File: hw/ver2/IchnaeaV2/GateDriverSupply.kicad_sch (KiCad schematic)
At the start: 0 parts

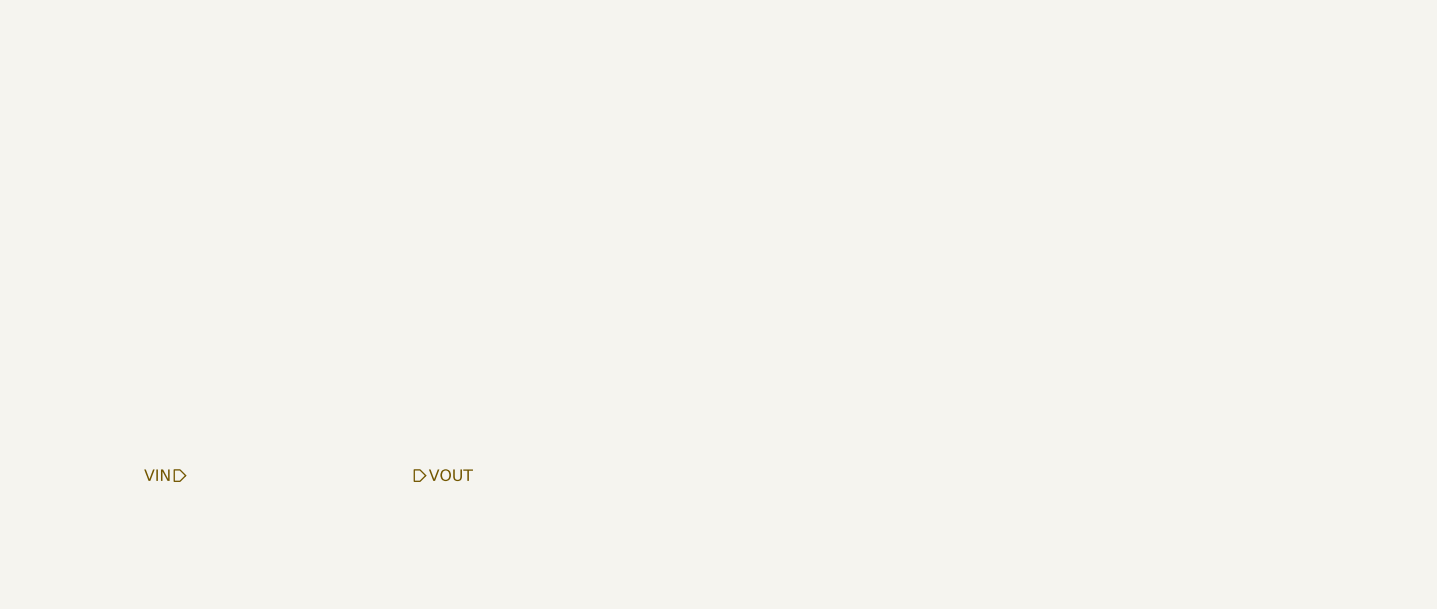
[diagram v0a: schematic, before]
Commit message: Sync work to main PC
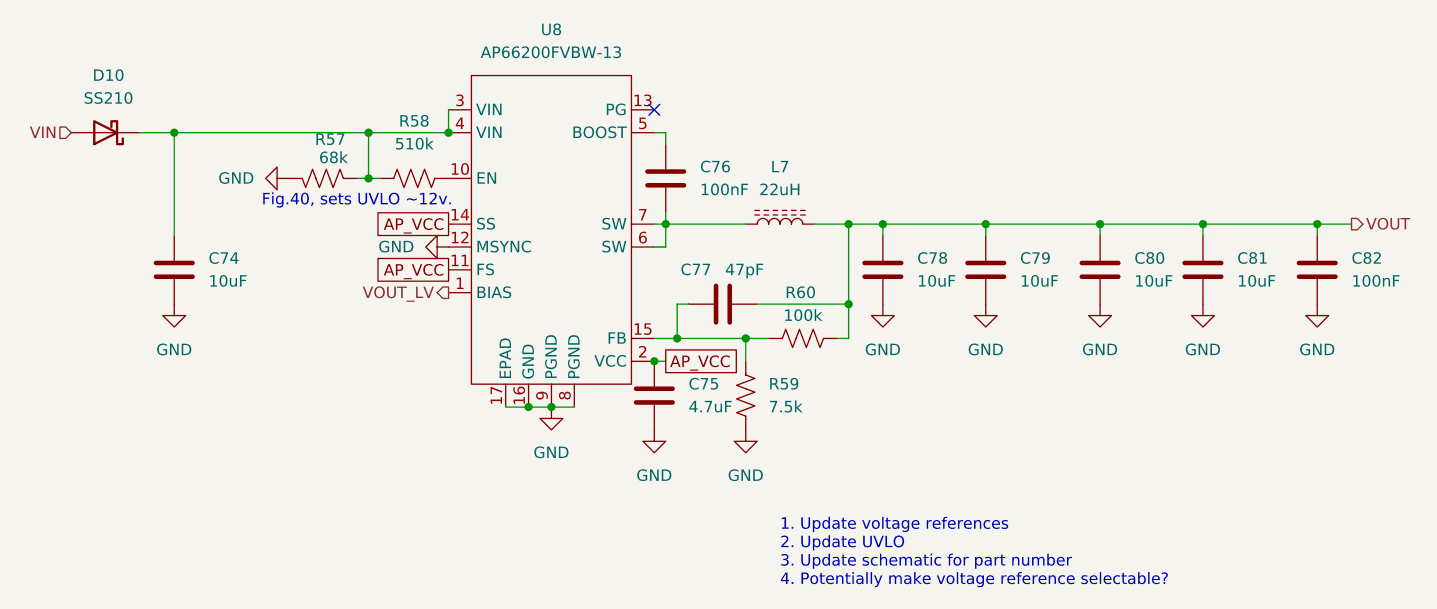
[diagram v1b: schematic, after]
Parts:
- added C74, C78, C79, C80, C81: 10uF, Capacitor_SMD:C_0603_1608Metric, symbol Device:C
- added C75: 4.7uF, Capacitor_SMD:C_0603_1608Metric, symbol Device:C
- added C76, C82: 100nF, Capacitor_SMD:C_0603_1608Metric, symbol Device:C
- added C77: 47pF, Capacitor_SMD:C_0603_1608Metric, symbol Device:C
- added D10: SS210, Diode_SMD:D_SMA, symbol Device:D_Schottky
- added L7: 22uH, Inductors:TYS5020220M, symbol Device:L_Ferrite
- added R57: 68k, Resistor_SMD:R_0603_1608Metric, symbol Device:R_US
- added R58: 510k, Resistor_SMD:R_0603_1608Metric, symbol Device:R_US
- added R59: 7.5k, Resistor_SMD:R_0603_1608Metric, symbol Device:R_US
- added R60: 100k, Resistor_SMD:R_0603_1608Metric, symbol Device:R_US
- added U8: AP66200FVBW-13, Package_DFN_QFN:QFN-16-1EP_4x4mm_P0.65mm_EP2.5x2.5mm, symbol ap66200:AP66200FVBW
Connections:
- net VIN: now also D10.2 (A)
- net VOUT: now also C77.2, C78.1, C79.1, C80.1, C81.1, C82.1, L7.2, R60.2
- new net: C74.1, D10.1 (K), R57.1, R58.1, U8.3 (VIN), U8.4 (VIN)
- new net: C76.1, U8.5 (BOOST)
- new net: C76.2, L7.1, U8.6 (SW), U8.7 (SW)
- new net: C77.1, R59.1, R60.1, U8.15 (FB)
- new net: R58.2, U8.10 (EN)
- new net AP_VCC: C75.1, U8.11 (FS), U8.14 (SS), U8.2 (VCC)
- new net GND: C74.2, C75.2, C78.2, C79.2, C80.2, C81.2, C82.2, R57.2, R59.2, U8.12 (MSYNC), U8.16 (GND), U8.17 (EPAD), U8.8 (PGND), U8.9 (PGND)
- new net VOUT_LV: U8.1 (BIAS)
- no-connect marks 0 -> 1
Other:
- note added: "1. Update voltage references 2. Update UVLO 3. Update schematic for part number 4. Potentially make voltage reference selectable?"
- note added: "Fig.40, sets UVLO ~12v."
